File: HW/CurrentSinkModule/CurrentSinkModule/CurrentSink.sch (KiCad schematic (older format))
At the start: 99 parts, among them J1 Conn_01x03, J2 Conn_01x03, J3 MosfetSocketx3, J4 MosfetSocketx3, U1 LTC2058, U2 LTC2058, U3 LTC2058, U4 LTC2058

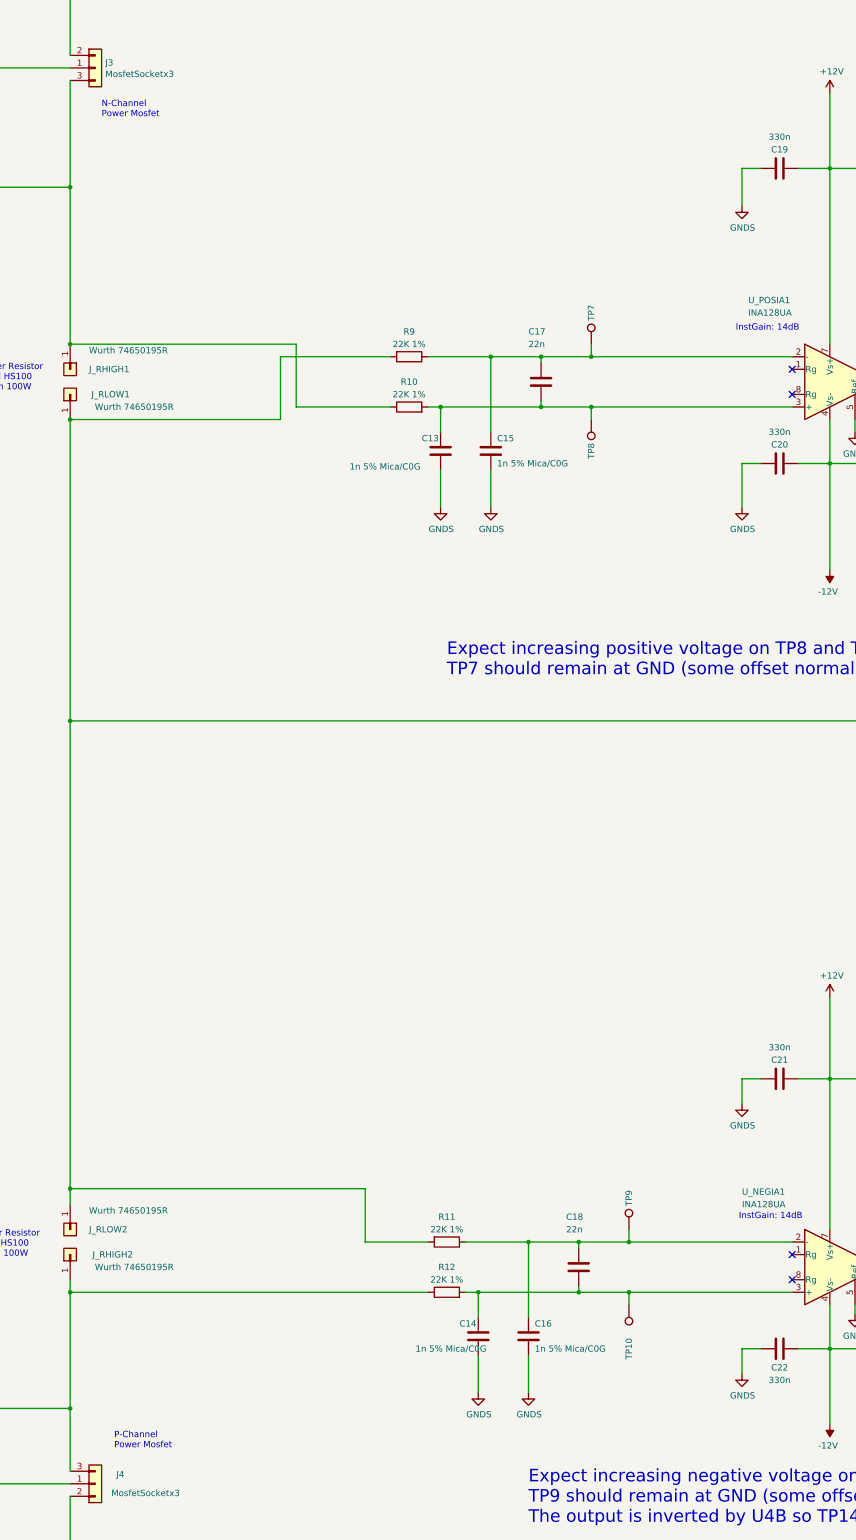
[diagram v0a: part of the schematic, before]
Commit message: updates
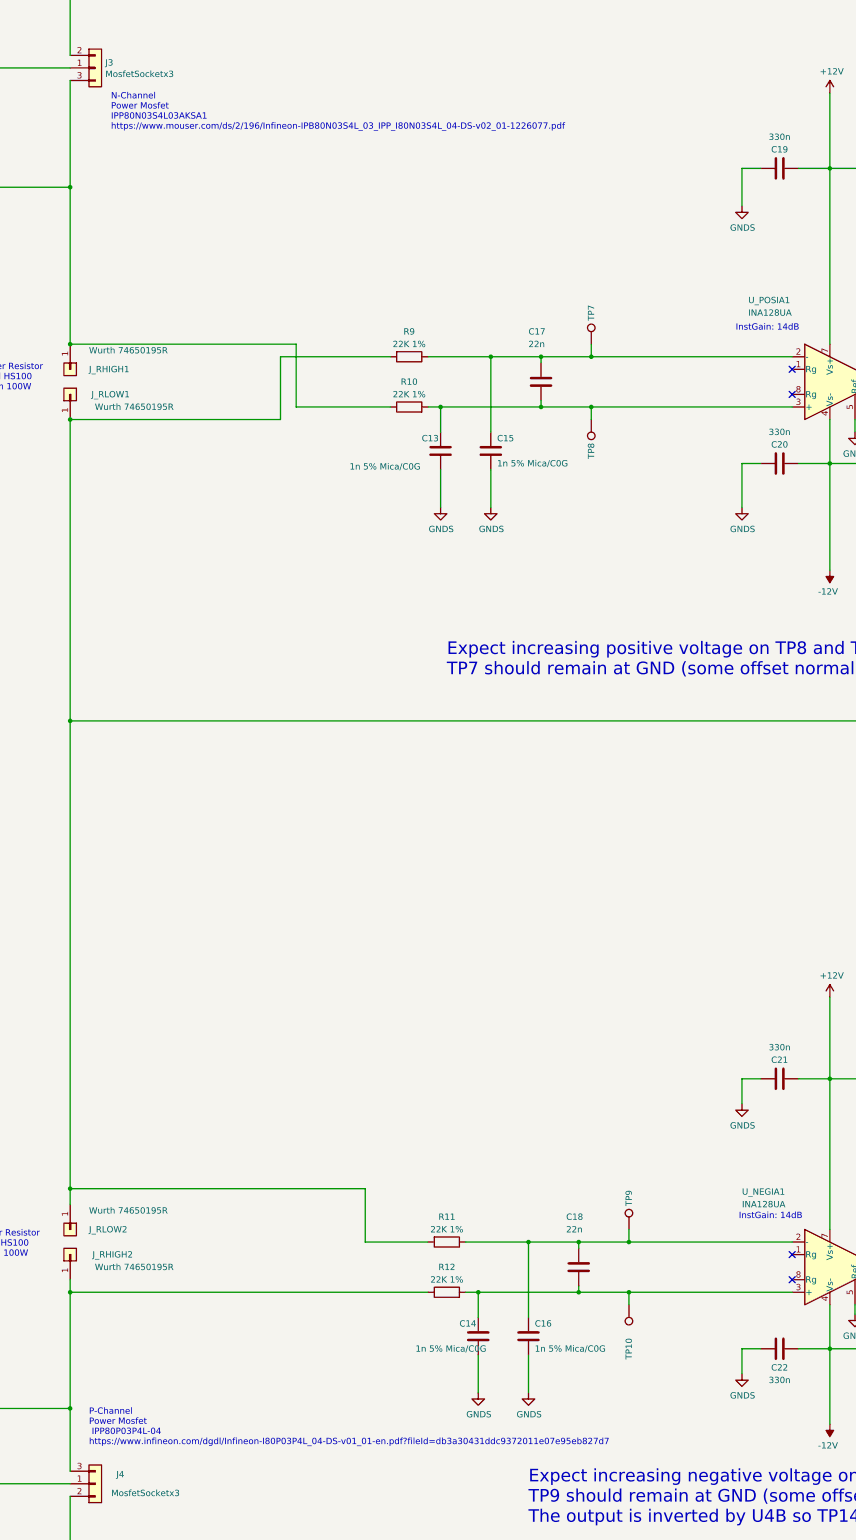
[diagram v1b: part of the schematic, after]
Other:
- note added: "N-Channel\nPower Mosfet\nIPP80N03S4L03AKSA1\nhttps://www.mouser.com/ds/2/196/Infineon-IPB80N03S4L_03_IPP_I80N03S4L_04-DS-v02_01-1226077.pdf"
- note added: "P-Channel\nPower Mosfet\n IPP80P03P4L-04\nhttps://www.infineon.com/dgdl/Infineon-I80P03P4L_04-DS-v01_01-en.pdf?fileId=db3a30431ddc9372011e07e95eb827d7"
- note removed: "N-Channel\nPower Mosfet"
- note removed: "P-Channel\nPower Mosfet"
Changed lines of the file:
@@
 Text Label 28900 8650 2    50   ~ 0
 DUT_POS
-Text Notes 14650 5050 0    50   ~ 0
-N-Channel\nPower Mosfet
+Text Notes 14725 5150 0    50   ~ 0
+N-Channel\nPower Mosfet\nIPP80N03S4L03AKSA1\nhttps://www.mouser.com/ds/2/196/Infineon-IPB80N03S4L_03_IPP_I80N03S4L_04-DS-v02_01-1226077.pdf
 Text Notes 13675 7225 0    50   ~ 0
 Power Resistor\nArcol HS100 \n1ohm 100W
-Text Notes 14750 15650 0    50   ~ 0
-P-Channel\nPower Mosfet
+Text Notes 14550 15625 0    50   ~ 0
+P-Channel\nPower Mosfet\n IPP80P03P4L-04\nhttps://www.infineon.com/dgdl/Infineon-I80P03P4L_04-DS-v01_01-en.pdf?fileId=db3a30431ddc9372011e07e95eb827d7
 Text Notes 19700 6750 0    50   ~ 0
 InstGain: 14dB
